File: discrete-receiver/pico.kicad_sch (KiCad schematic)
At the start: 44 parts, among them SW1 Reset, U12 TPS7A20xxxDBV, U13 LM66100DCK, U14 LM66100DCK, U15 LM66100DCK, U6 RP2350A, U7 W25Q128JVS, U8 NCP1117-3.3_SOT223, Y1 ABM8-272-T3

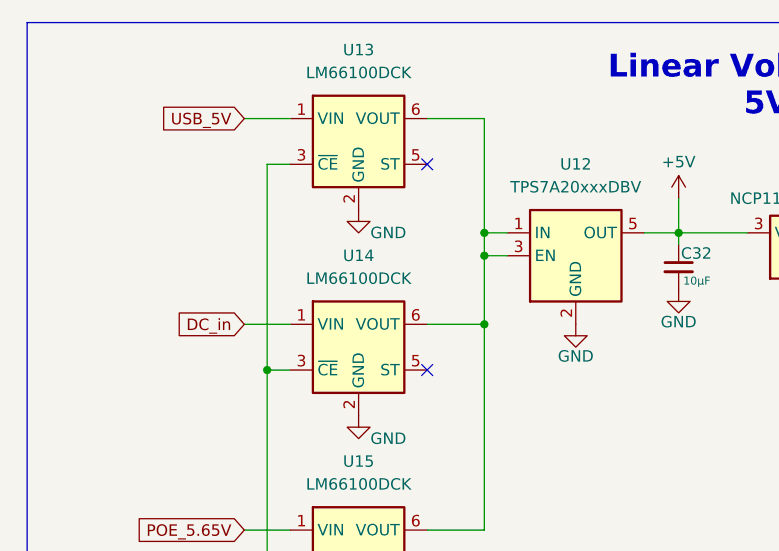
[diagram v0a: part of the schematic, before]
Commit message: Fixed a couple bugs
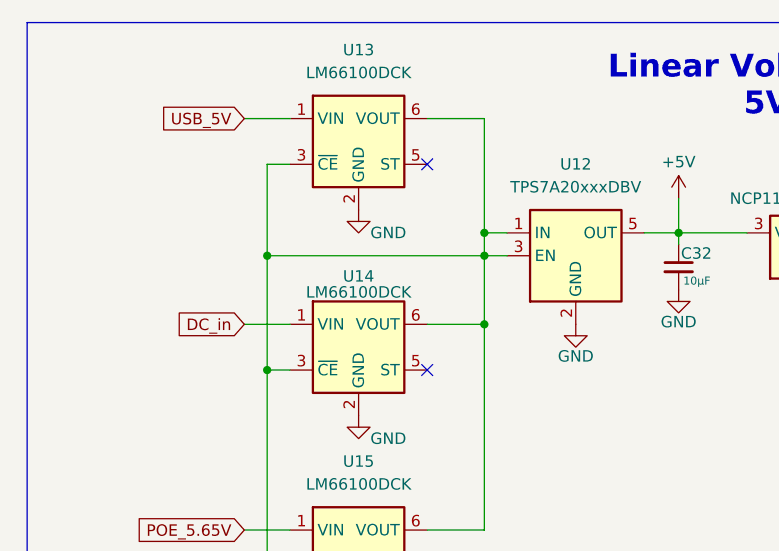
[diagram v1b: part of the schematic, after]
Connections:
- net at U13.3 (~{CE}), U14.3 (~{CE}), U15.3 (~{CE}): now also U12.1 (IN), U12.3 (EN), U13.6 (VOUT), U14.6 (VOUT), U15.6 (VOUT)
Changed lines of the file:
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@@
+	)
+	(junction
+		(at 41.91 40.64)
+		(diameter 0)
+		(color 0 0 0 0)
 	)
 	(junction
@@
 	(wire
 		(pts
+			(xy 41.91 40.64) (xy 41.91 53.34)
+		)
+		(stroke
+			(width 0)
+			(type default)
+		)
+	)
+	(wire
+		(pts
 			(xy 171.45 33.02) (xy 179.07 33.02)
 		)
@@
 	(wire
 		(pts
+			(xy 41.91 40.64) (xy 66.04 40.64)
+		)
+		(stroke
+			(width 0)
+			(type default)
+		)
+	)
+	(wire
+		(pts
 			(xy 191.77 66.04) (xy 191.77 52.07)
 		)
@@
 	(wire
 		(pts
-			(xy 41.91 30.48) (xy 41.91 53.34)
+			(xy 41.91 30.48) (xy 41.91 40.64)
 		)
 		(stroke
@@
 		(in_pos_files yes)
 		(dnp no)
-		(fields_autoplaced yes)
 		(property "Reference" "U14"
-			(at 52.07 40.64 0)
+			(at 52.07 42.926 0)
 			(show_name no)
 			(do_not_autoplace no)
@@
 		)
 		(property "Value" "LM66100DCK"
-			(at 52.07 43.18 0)
-			(show_name no)
-			(do_not_autoplace no)
+			(at 52.07 44.704 0)
+			(show_name no)
+			(do_not_autoplace no)
